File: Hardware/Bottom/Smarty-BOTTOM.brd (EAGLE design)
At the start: 160 x 100 mm, 0 parts

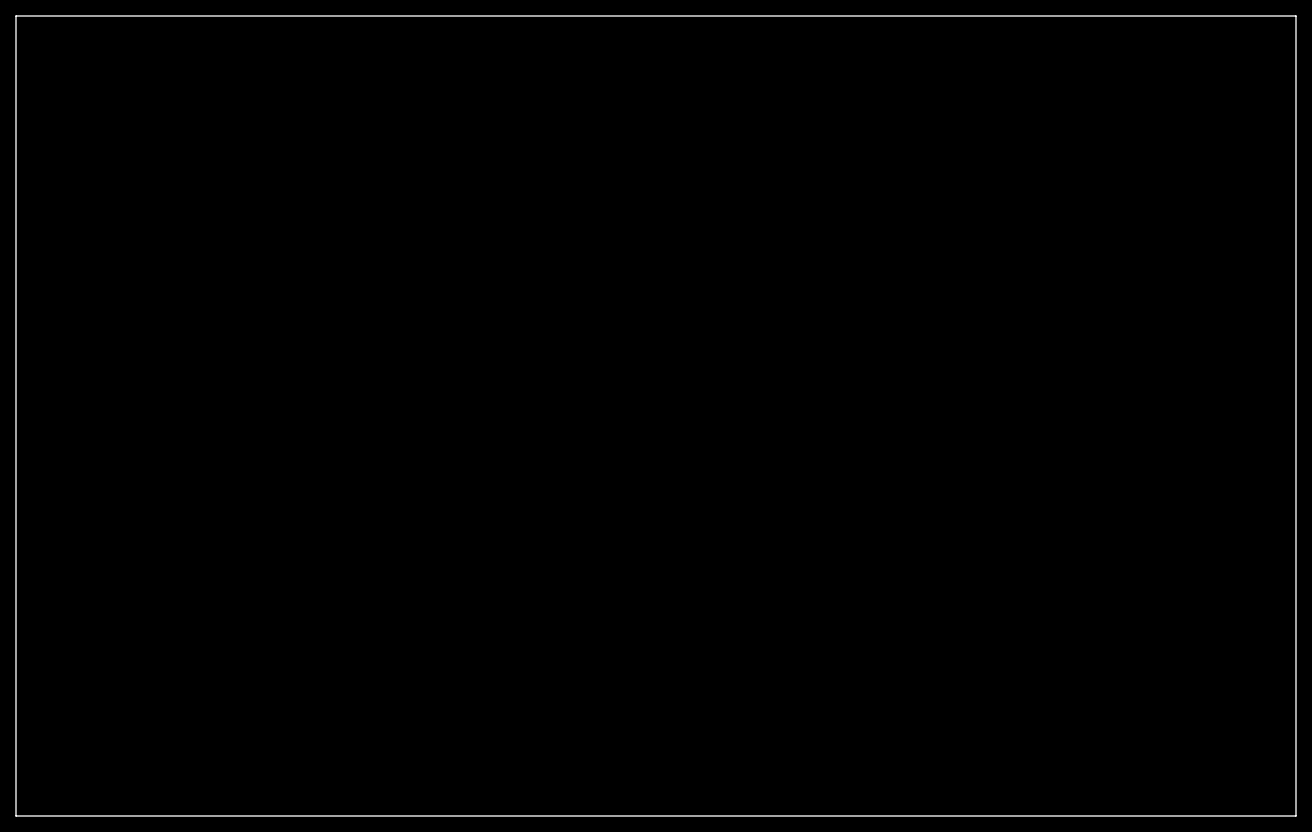
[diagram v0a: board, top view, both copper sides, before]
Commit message: Take 001 and part of Take 002 Completed
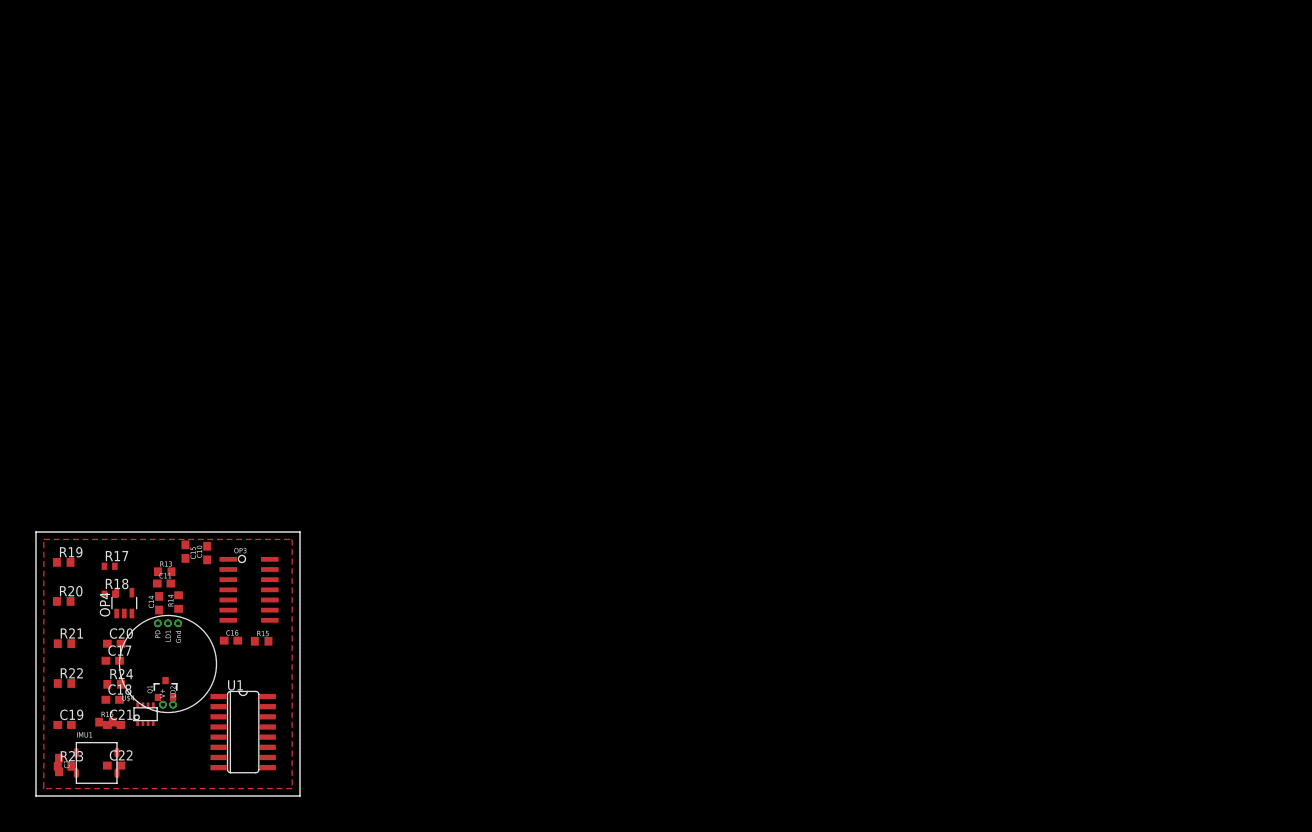
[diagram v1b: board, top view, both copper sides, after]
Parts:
- added C1, C10, C11, C17, C18, C22: 100n, LinnesLab-Passives:C0603
- added C14, C19: 2.2n, LinnesLab-Passives:C0603
- added C15, C16: 2.2u, LinnesLab-Passives:C0603
- added C20: 22u, LinnesLab-Passives:C0603
- added C21: 22n, LinnesLab-Passives:C0603
- added IMU1: LSM6DS3_CAST, LinnesLab-Sensors:LSM6DS3_CAST
- added OP3: (no value), LinnesLab-AnalogIC:SO14
- added OP4: (no value), LinnesLab-AnalogIC:SOT23-5
- added Q1: (no value), LinnesLab-DiscreteSemi:SOT23-3
- added R13, R15, R19, R21: 220k, LinnesLab-Passives:R0603
- added R14, R22: 10M, LinnesLab-Passives:R0603
- added R16: (no value), LinnesLab-Passives:R0603
- added R17, R18: 10k, LinnesLab-Passives:R0402
- added R20, R23: 1M, LinnesLab-Passives:R0603
- added R24: 10k, LinnesLab-Passives:R0603
- added U$3: (no value), LinnesLab-Connectors:PPG.MODULE.2
- added U$4: AD5171, LinnesLab-DigitalIC:SOT-23-8
- added U1: AD5242-SO16, LinnesLab-DigitalIC:SO16
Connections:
- new net 3.3V: C1.2, C11.2, C17.2, C18.2, C22.2, IMU1.2, OP3.4, OP4.5, R13.2, R15.2, R17.2, U$3.V+, U$4.2, U$4.6, U1.5, U1.6
- new net G.A1: U1.2
- new net G.A2: U1.16
- new net G.O1: U1.1
- new net G.O2: U1.13
- new net G.W2: C21.1, OP3.2, R24.1, U1.15
- new net GND: C1.1, C11.1, C17.1, C18.1, C22.1, IMU1.1, OP3.11, OP4.2, OP4.3, Q1.2, R18.1, R19.1, R21.1, U$3.GND, U$4.3, U1.10, U1.11, U1.12, U1.9
- new net LED: Q1.3
- new net LED.C: U$3.LD1
- new net LED.CTRL: U$4.8
- new net N$10: OP3.12, R17.1, R18.2
- new net N$13: C15.2, OP3.5, R13.1, R19.2
- new net N$15: C14.2, OP3.6, R14.1, R20.2
- new net N$16: C14.1, C16.1, OP3.7, R14.2
- new net N$17: C16.2, OP3.10, R15.1, R21.2
- new net N$18: C19.2, OP3.9, R22.1, R23.2
- new net N$19: C19.1, C20.1, OP3.8, R22.2
- new net N$20: C20.2, R24.2
- new net N$8: Q1.1, R16.2
- new net N$9: R16.1, U$4.1, U$4.7
- new net PD.C: C10.1, OP4.4, U$3.PD, U1.4
- new net PPG: C21.2, OP3.1, U1.14
- new net SCL: IMU1.3, U$4.4, U1.7
- new net SDA: IMU1.4, U$4.5, U1.8
- new net TIA: C10.2, C15.1, OP4.1, U1.3
- new net VREF: OP3.13, OP3.14, OP3.3, R20.1, R23.1
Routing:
- added copper zone on layer 1, net 3.3V
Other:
- board size 160 x 100 mm -> 33 x 33 mm
